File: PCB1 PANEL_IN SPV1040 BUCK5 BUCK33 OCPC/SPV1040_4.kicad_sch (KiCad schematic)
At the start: 14 parts, among them J5 SOLAR, U5 SPV1040TTR

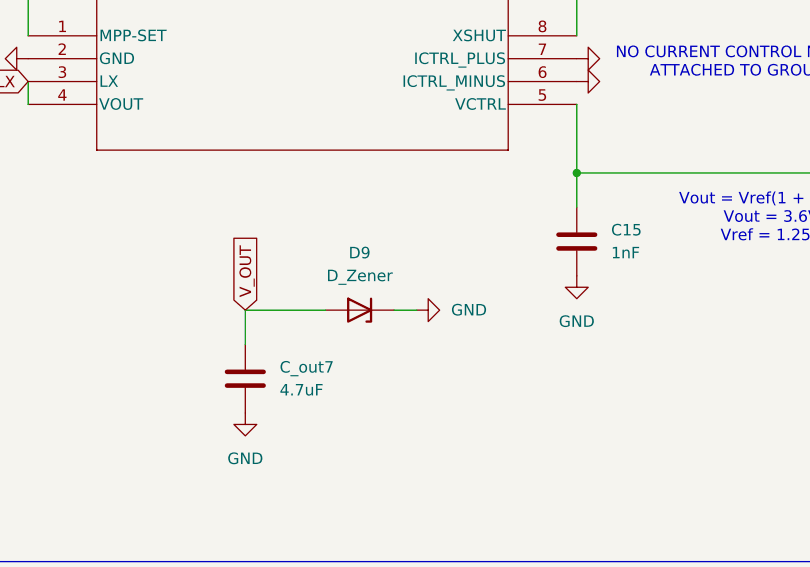
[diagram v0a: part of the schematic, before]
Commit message: w
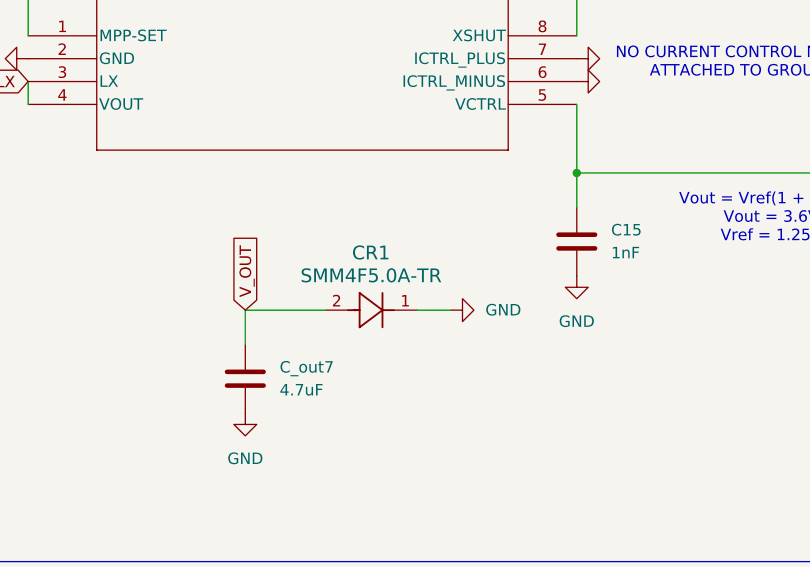
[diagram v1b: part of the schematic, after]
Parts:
- removed D9: D_Zener, Diode_SMD:D_1210_3225Metric, symbol Device:D_Zener
- added CR1: SMM4F5.0A-TR, CR_F5.0A-TR_STM, symbol SMM4F5:SMM4F5.0A-TR
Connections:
- net GND: now also CR1.1
- net PANEL1_OUT: now also CR1.2
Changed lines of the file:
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@@
+	(wire
+		(pts
+			(xy 93.98 105.41) (xy 97.79 105.41)
+		)
+		(stroke
+			(width 0)
+			(type default)
+		)
+	)
 	(wire
 		(pts
@@
 		(pts
 			(xy 231.14 96.52) (xy 245.11 96.52)
-		)
-		(stroke
-			(width 0)
-			(type default)
-		)
-	)
-	(wire
-		(pts
-			(xy 91.44 105.41) (xy 93.98 105.41)
 		)
 		(stroke
@@
 	)
 	(symbol
-		(lib_id "Device:D_Zener")
-		(at 87.63 105.41 180)
-		(unit 1)
-		(exclude_from_sim no)
-		(in_bom yes)
-		(on_board yes)
-		(dnp no)
-		(fields_autoplaced yes)
-		(property "Reference" "D9"
-			(at 87.63 99.06 0)
-			(effects
-				(font
-					(size 1.27 1.27)
-				)
-			)
-		)
-		(property "Value" "D_Zener"
-			(at 87.63 101.6 0)
-			(effects
-				(font
-					(size 1.27 1.27)
-				)
-			)
-		)
-		(property "Footprint" "Diode_SMD:D_1210_3225Metric"
-			(at 87.63 105.41 0)
-			(effects
-				(font
-					(size 1.27 1.27)
-				)
-				(hide yes)
-			)
-		)
-		(property "Datasheet" "~"
-			(at 87.63 105.41 0)
-			(effects
-				(font
-					(size 1.27 1.27)
-				)
-				(hide yes)
-			)
-		)
-		(property "Description" "Zener diode"
-			(at 87.63 105.41 0)
-			(effects
-				(font
-					(size 1.27 1.27)
-				)
-				(hide yes)
-			)
-		)
-		(pin "2"
-		)
-		(pin "1"
-		)
-		(instances
-			(project "PCB1 PANEL_IN SPV1040 BUCK5 BUCK33 OCPC"
-				(path "/494c9d9f-6b33-4248-a813-27ffaaa929bd/2771644a-42c1-4e74-9e93-0ffcf5523547"
-					(reference "D9")
-					(unit 1)
-				)
-			)
-		)
-	)
-	(symbol
 		(lib_id "power:GND")
 		(at 111.76 101.6 0)
@@
 	(symbol
 		(lib_id "power:GND")
-		(at 93.98 105.41 90)
+		(at 97.79 105.41 90)
 		(unit 1)
 		(exclude_from_sim no)
@@
 		(fields_autoplaced yes)
 		(property "Reference" "#PWR046"
-			(at 100.33 105.41 0)
+			(at 104.14 105.41 0)
 			(effects
 				(font
@@
 		)
 		(property "Value" "GND"
-			(at 97.79 105.4099 90)
+			(at 101.6 105.4099 90)
 			(effects
 				(font
@@
 		)
 		(property "Footprint" ""
-			(at 93.98 105.41 0)
+			(at 97.79 105.41 0)
 			(effects
 				(font
@@
 		)
 		(property "Datasheet" ""
-			(at 93.98 105.41 0)
+			(at 97.79 105.41 0)
 			(effects
 				(font
@@
 		)
 		(property "Description" "Power symbol creates a global label with name \"GND\" , ground"
-			(at 93.98 105.41 0)
+			(at 97.79 105.41 0)
 			(effects
 				(font
@@
 					(unit 1)
 				)
+			)
+		)
+	)
+	(symbol
+		(lib_id "SMM4F5:SMM4F5.0A-TR")
+		(at 83.82 105.41 0)
+		(unit 1)
+		(exclude_from_sim no)
+		(in_bom yes)
+		(on_board yes)
+		(dnp no)
+		(fields_autoplaced yes)
+		(property "Reference" "CR1"
+			(at 88.9 99.06 0)
+			(effects
+				(font
+					(size 1.524 1.524)
+				)
+			)
+		)
+		(property "Value" "SMM4F5.0A-TR"
+			(at 88.9 101.6 0)
+			(effects
+				(font
+					(size 1.524 1.524)
+				)
+			)
+		)
+		(property "Footprint" "CR_F5.0A-TR_STM"
+			(at 83.82 105.41 0)
+			(effects
+				(font
+					(size 1.27 1.27)
+					(italic yes)
+				)
+				(hide yes)
+			)
+		)
+		(property "Datasheet" "SMM4F5.0A-TR"
+			(at 83.82 105.41 0)
+			(effects
+				(font
+					(size 1.27 1.27)
+					(italic yes)
+				)
+				(hide yes)
+			)
+		)
+		(property "Description" ""
+			(at 83.82 105.41 0)
+			(effects
+				(font
+					(size 1.27 1.27)
+				)
+				(hide yes)
+			)
+		)
+		(pin "1"
+		)
+		(pin "2"
+		)
+		(instances
+			(project ""
+				(path "/494c9d9f-6b33-4248-a813-27ffaaa929bd/2771644a-42c1-4e74-9e93-0ffcf5523547"
+					(reference "CR1")
+					(unit 1)
+				)
